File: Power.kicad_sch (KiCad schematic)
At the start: 29 parts, among them IC1 ADP2301AUJZ-R7, IC2 ADP2301AUJZ-R7, J8 Conn_01x02, Q1 AO3401A, U1 LM2842X, U6 XT30PW-F, U7 XT30PW-M

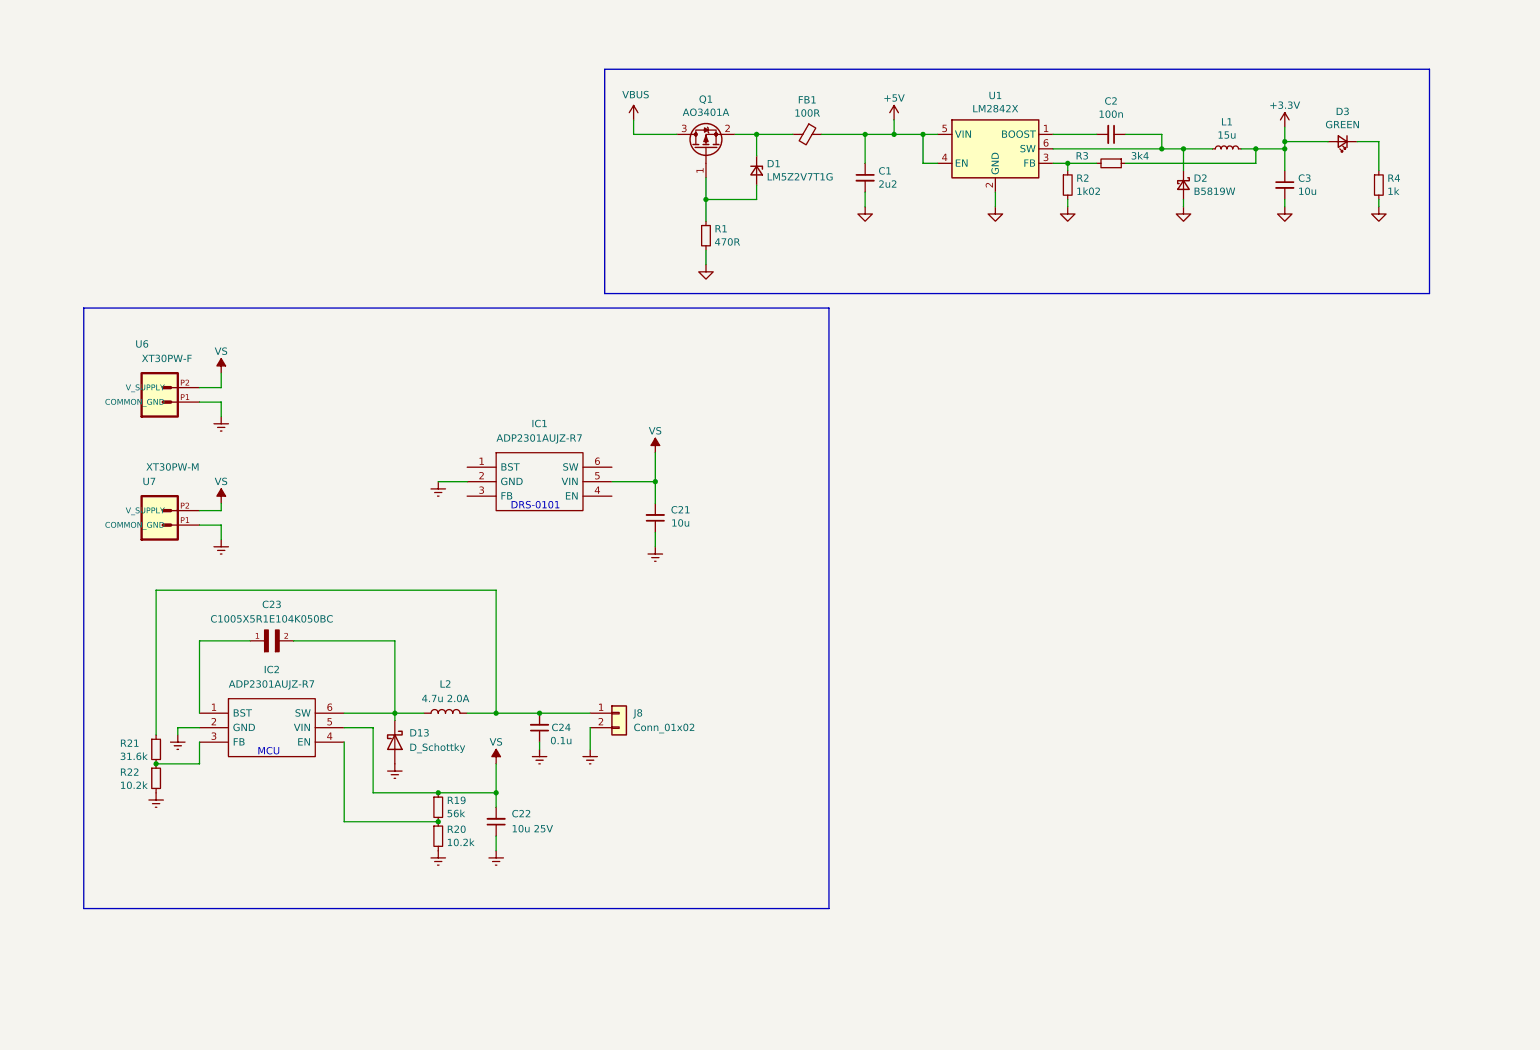
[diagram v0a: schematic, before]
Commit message: skgnigniogni
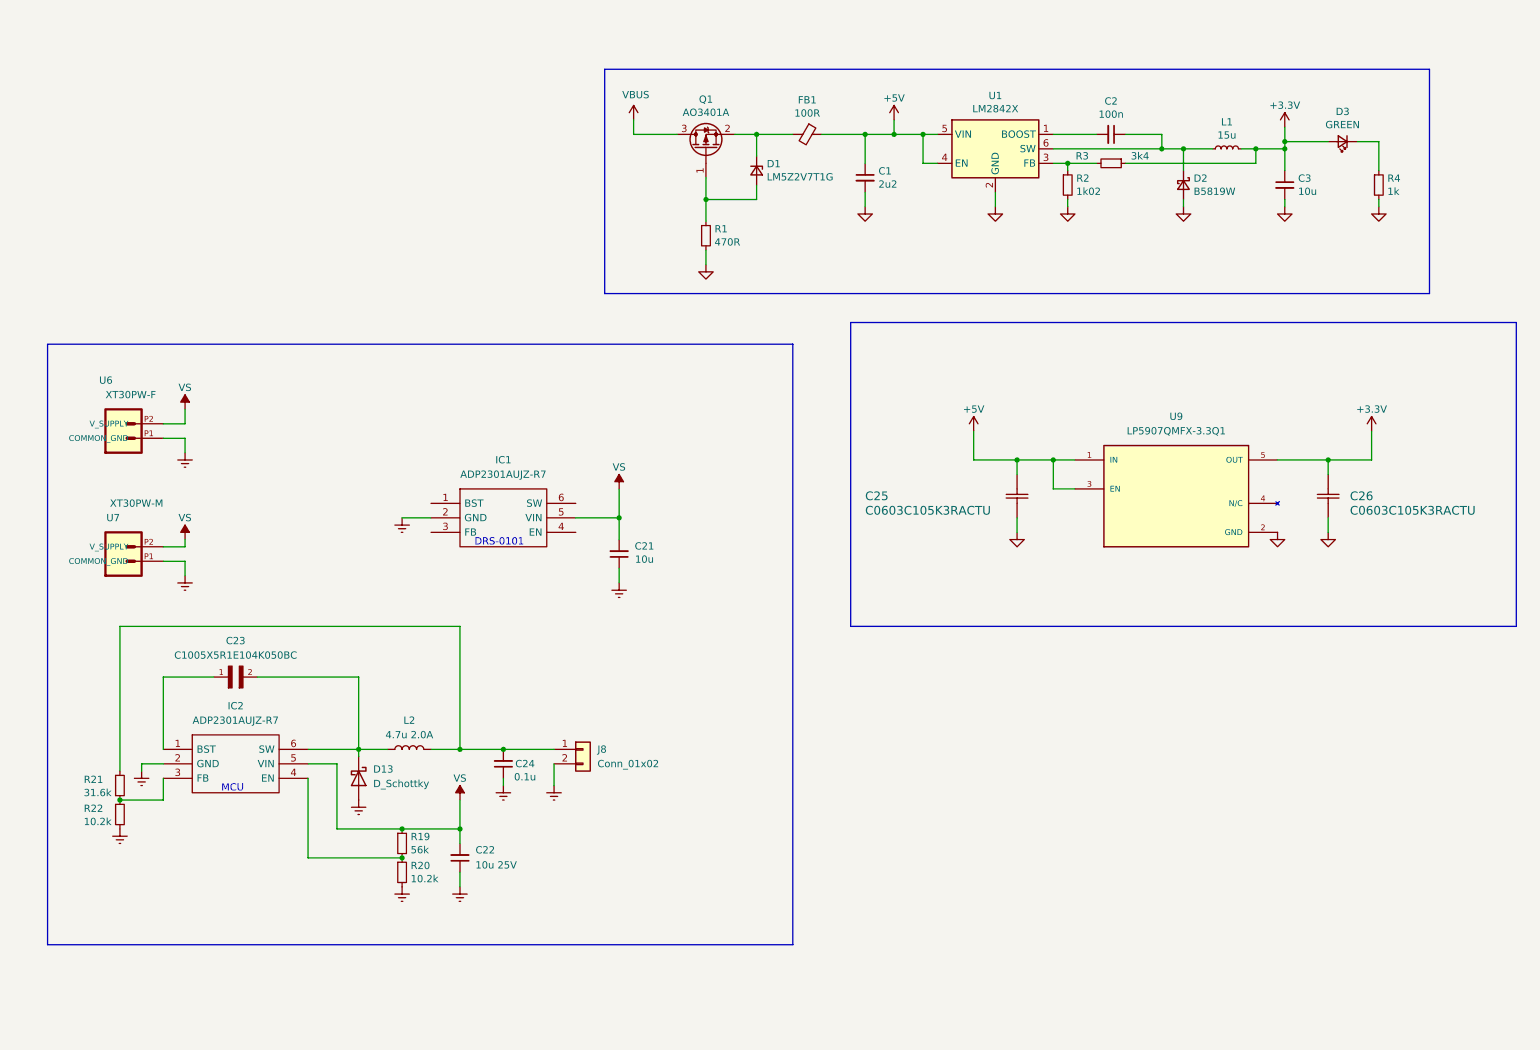
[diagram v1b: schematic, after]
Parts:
- added C25, C26: C0603C105K3RACTU, SnapEDA Library:C0603C105K3RACTU, symbol C0603C105K3RACTU:C0603C105K3RACTU
- added U9: LP5907QMFX-3.3Q1, SnapEDA Library:SOT95P280X145-5N, symbol LP5907QMFX-3.3Q1:LP5907QMFX-3.3Q1
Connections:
- net +3V3: now also C26.2, U9.5 (OUT)
- net +5V: now also C25.2, U9.1 (IN), U9.3 (EN)
- net GND: now also C25.1, C26.1, U9.2 (GND)
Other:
- moved on the sheet: C21, C22, C23, C24, D13, IC1, IC2, J8, L2, R19, R20, R21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

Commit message: sgsegwaebdd
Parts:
- J8: footprint SnapEDA Library:JST_BM02B-SURS-TF(LF)(SN) -> (none)
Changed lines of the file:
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@@
     (pin "6")
-  )
-  (symbol (lib_id "Connector_Generic:Conn_01x02") (at 116.84 144.78 0) (unit 1)
-    (in_bom yes) (on_board yes) (fields_autoplaced)
-    (property "Reference" "J8" (id 0) (at 119.38 144.7799 0)
-      (effects (font (size 1.27 1.27)) (justify left))
-    )
-    (property "Value" "Conn_01x02" (id 1) (at 119.38 147.3199 0)
-      (effects (font (size 1.27 1.27)) (justify left))
-    )
-    (property "Footprint" "SnapEDA Library:JST_BM02B-SURS-TF(LF)(SN)" (id 2) (at 116.84 144.78 0)
-      (effects (font (size 1.27 1.27)) hide)
-    )
-    (property "Datasheet" "~" (id 3) (at 116.84 144.78 0)
-      (effects (font (size 1.27 1.27)) hide)
-    )
-    (pin "1")
-    (pin "2")
   )
   (symbol (lib_id "power:Earth") (at 111.76 151.13 0) (unit 1)
@@
       (effects (font (size 1.27 1.27)) hide)
     )
+    (pin "1")
+    (pin "2")
+  )
+  (symbol (lib_id "Connector_Generic:Conn_01x02") (at 116.84 144.78 0) (unit 1)
+    (in_bom yes) (on_board yes) (fields_autoplaced)
+    (property "Reference" "J8" (id 0) (at 119.38 144.7799 0)
+      (effects (font (size 1.27 1.27)) (justify left))
+    )
+    (property "Value" "Conn_01x02" (id 1) (at 119.38 147.3199 0)
+      (effects (font (size 1.27 1.27)) (justify left))
+    )
+    (property "Footprint" "" (id 2) (at 116.84 144.78 0)
+      (effects (font (size 1.27 1.27)) hide)
+    )
+    (property "Datasheet" "~" (id 3) (at 116.84 144.78 0)
+      (effects (font (size 1.27 1.27)) hide)
+    )

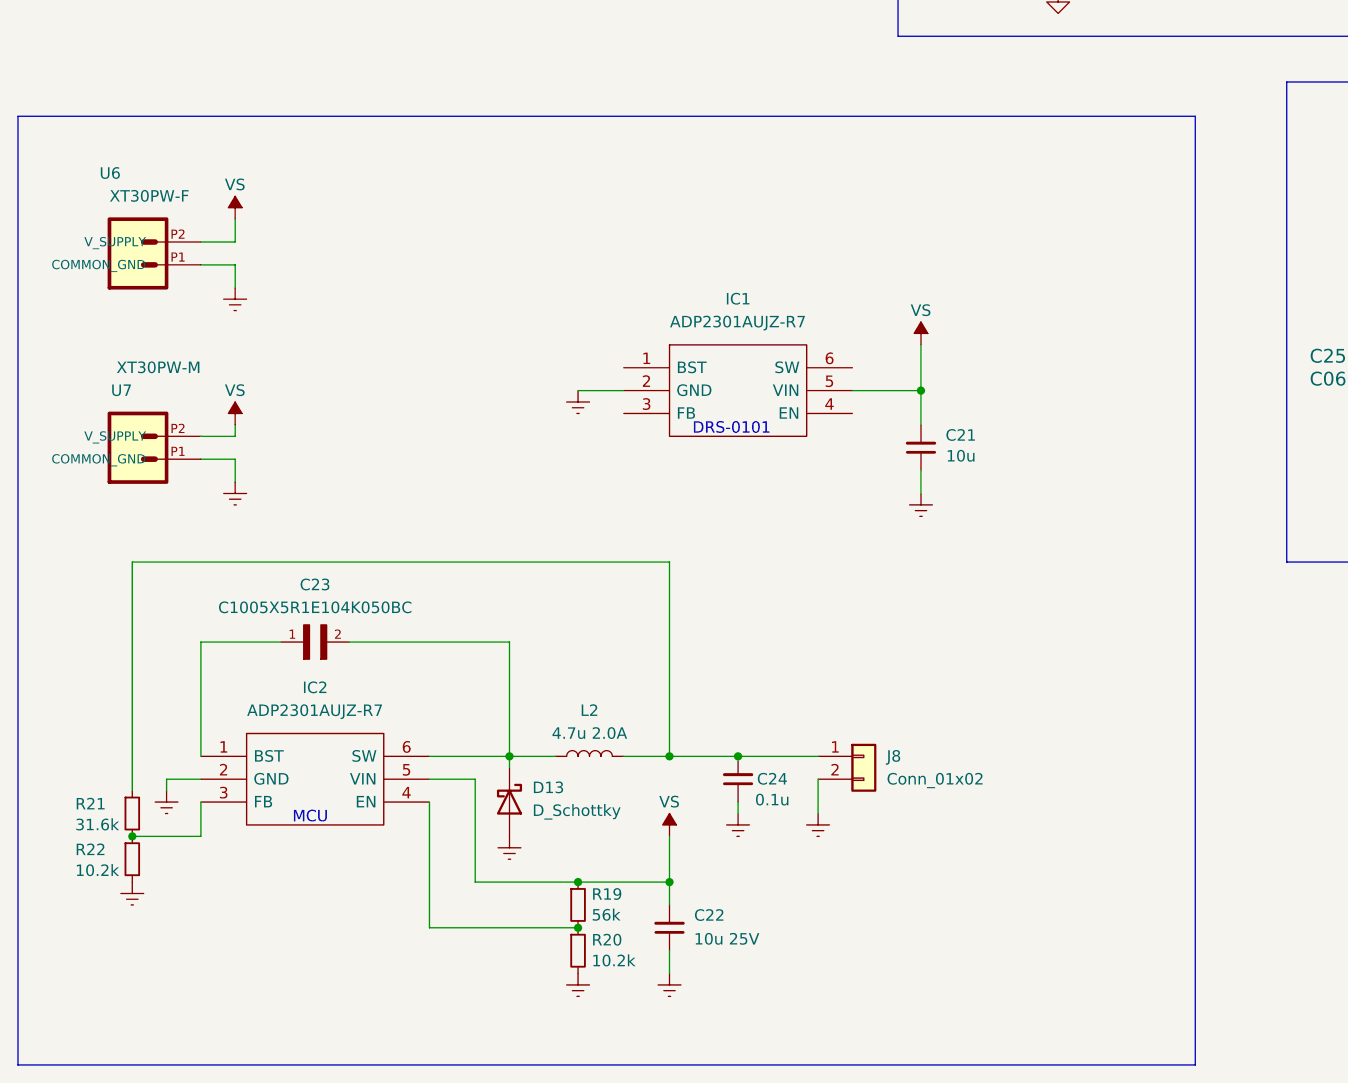
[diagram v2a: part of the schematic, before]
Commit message: sdgionbidnb
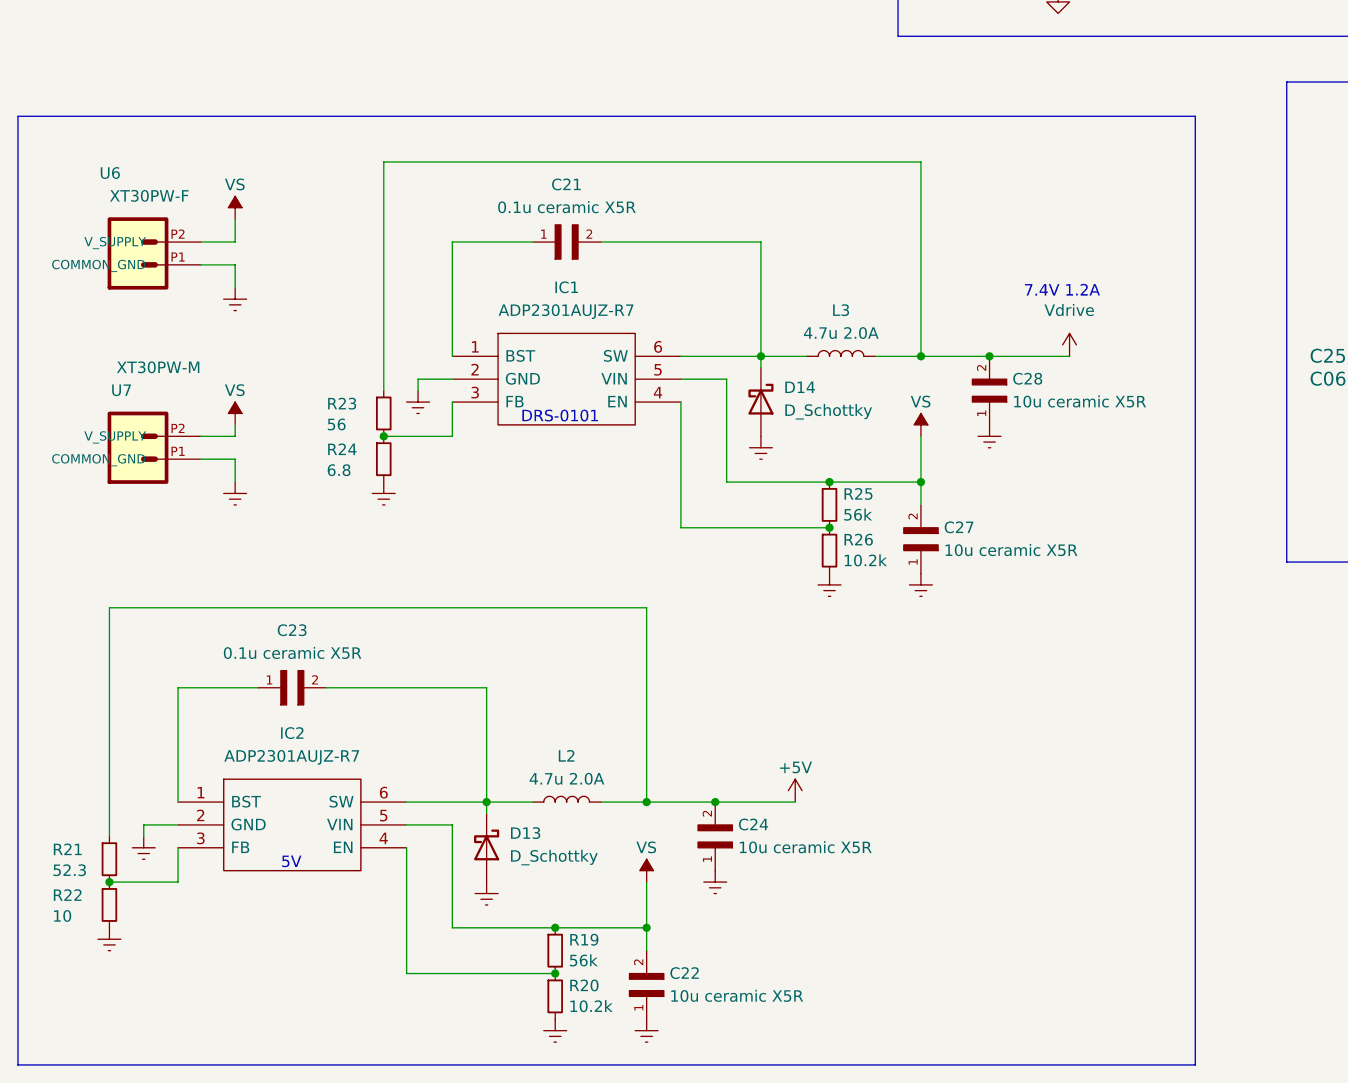
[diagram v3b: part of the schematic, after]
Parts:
- removed C21: 10u, Capacitor_SMD:C_0402_1005Metric, symbol Device:C_Small
- removed C22: 10u 25V, Capacitor_SMD:C_0402_1005Metric, symbol Device:C_Small
- removed C24: 0.1u, Capacitor_SMD:C_0402_1005Metric, symbol Device:C_Small
- removed J8: Conn_01x02, symbol Connector_Generic:Conn_01x02
- added C21: 0.1u ceramic X5R, SnapEDA Library:CAPC1005X55N, symbol C1005X5R1E104K050BC:C1005X5R1E104K050BC
- added C22, C24, C27, C28: 10u ceramic X5R, SnapEDA Library:CAPC1608X90N, symbol C1608X5R0J106K080AB:C1608X5R0J106K080AB
- added D14: D_Schottky, SnapEDA Library:B230A-13-F, symbol Device:D_Schottky
- added L3: 4.7u 2.0A, SnapEDA Library:CDRH5D28RHPNP-4R7NC, symbol Device:L
- added R23: 56, Resistor_SMD:R_0402_1005Metric, symbol Device:R_Small
- added R24: 6.8, Resistor_SMD:R_0402_1005Metric, symbol Device:R_Small
- added R25: 56k, Resistor_SMD:R_0402_1005Metric, symbol Device:R_Small
- added R26: 10.2k, Resistor_SMD:R_0402_1005Metric, symbol Device:R_Small
- C23: value C1005X5R1E104K050BC -> 0.1u ceramic X5R
- R21: value 31.6k -> 52.3
- R22: value 10.2k -> 10
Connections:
- net +5V: now also L2.2, R21.1, C24.2
- net Earth: now also C22.1, C24.1, C27.1, C28.1, D14.2 (A), R24.2, R26.2
- net VS: now also C22.2, C27.2, R25.1
- net at IC1.1 (BST): now also C21.1
- net at IC1.3 (FB): now also R23.2, R24.1
- net at IC1.4 (EN): now also R25.2, R26.1
- net at IC1.6 (SW): now also C21.2, D14.1 (K), L3.1
- new net Vdrive: C28.2, L3.2, R23.1
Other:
- note added: "5V"
- note added: "7.4V 1.2A"
- note removed: "MCU"
- moved on the sheet: C23, D13, IC1, IC2, L2, R19, R20, R21, R22
